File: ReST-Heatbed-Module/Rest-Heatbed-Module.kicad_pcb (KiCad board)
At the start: 2 copper layers, 25.4 x 34.2 mm, 88 parts, among them P1 02-SCREW-TERM, P2 CONN_02X03, P3 02-SCREW-TERM, P4 01X02-MALE, P5 02-SCREW-TERM, Q1 Q_BSH105, Q2 Q_AOT240L

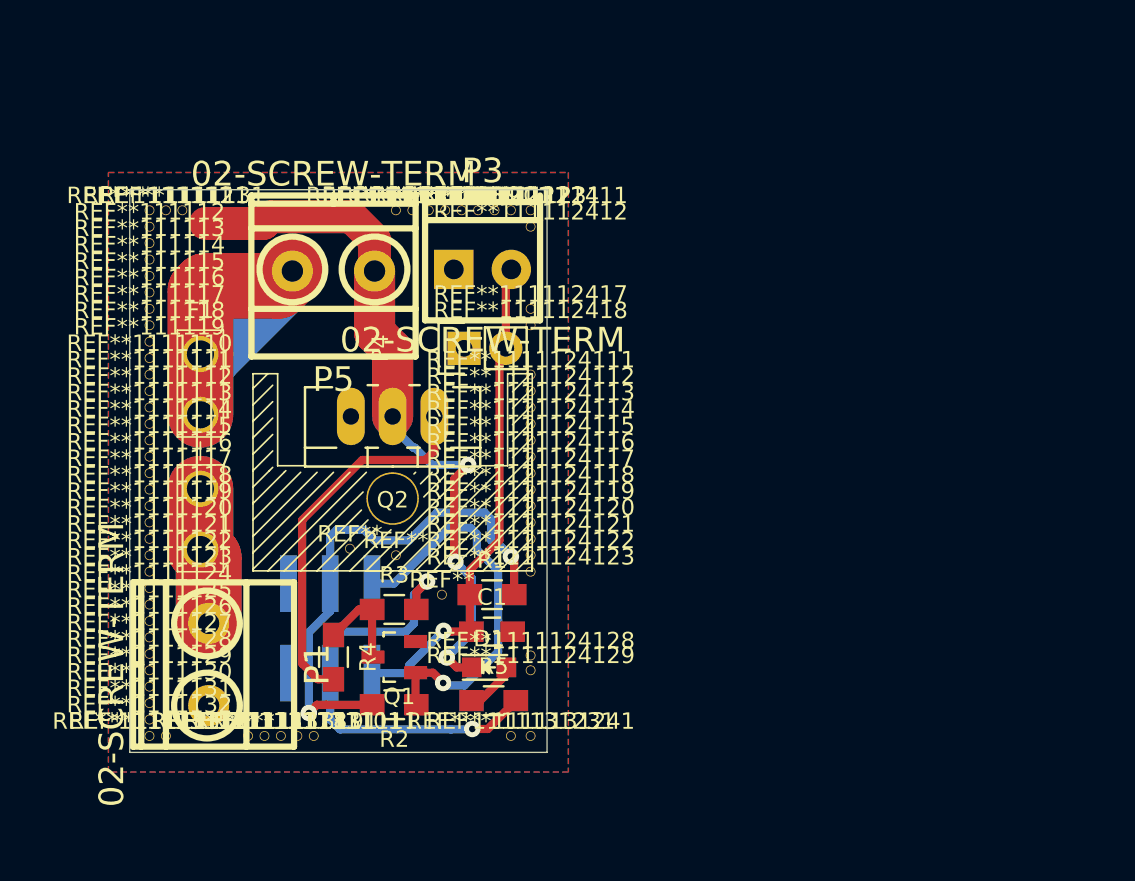
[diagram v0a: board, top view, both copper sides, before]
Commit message: Mainboard structure made and most modules finished
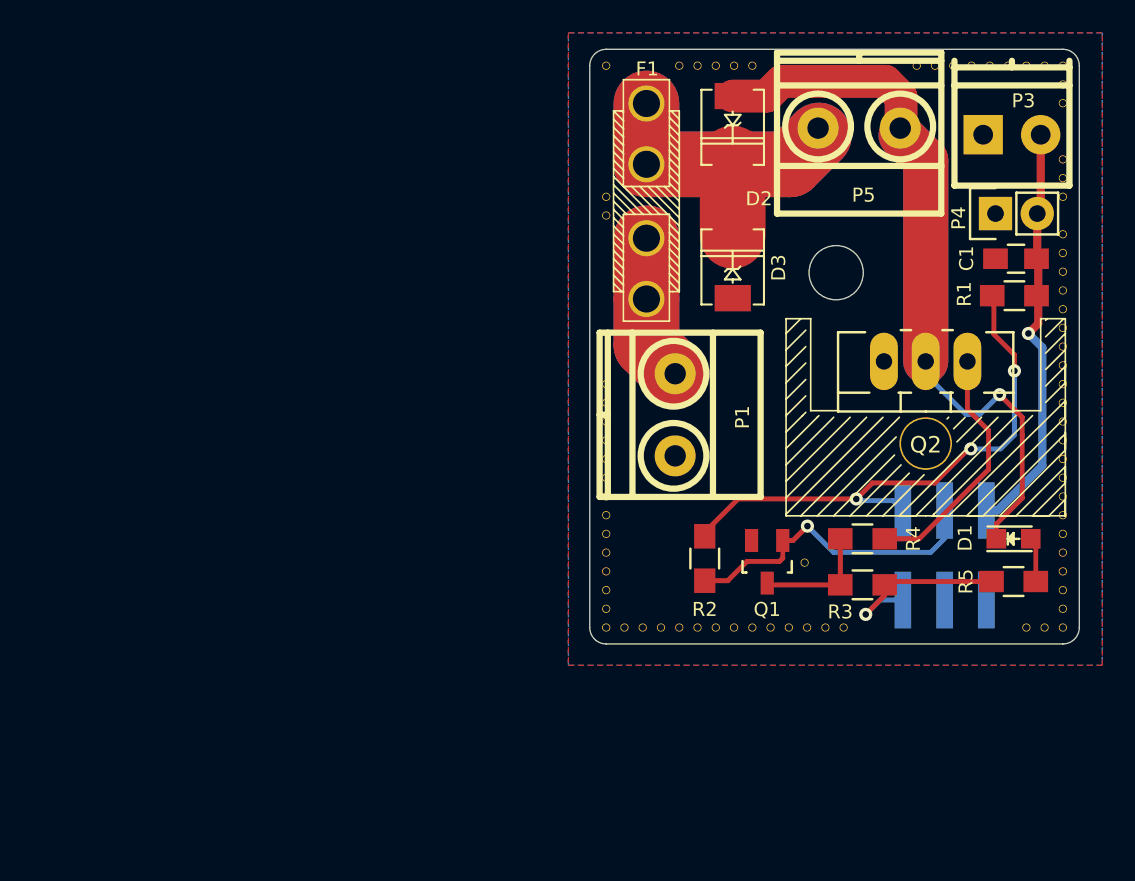
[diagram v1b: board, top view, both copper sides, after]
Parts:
- removed REF** (x3), REF**1111110, REF**1111111 (x2), REF**1111112, REF**1111113, REF**1111114, REF**1111115, REF**1111116, REF**1111117, REF**11111171 (x2), REF**1111118, REF**11111181, REF**1111119, REF**11111191, REF**111112, REF**1111120, REF**11111201, REF**1111121 (x2), REF**11111211, REF**1111122, REF**11111221, REF**1111123, REF**11111231, REF**1111124, REF**111112411, REF**1111124111, REF**1111124112, REF**1111124113, REF**1111124114, REF**1111124115, REF**1111124116, REF**1111124117, REF**1111124118, REF**1111124119, REF**111112412, REF**1111124120, REF**1111124121, REF**1111124122, REF**1111124123, REF**1111124128, REF**1111124129, REF**111112417, REF**111112418, REF**1111125, REF**1111126, REF**1111127, REF**1111128, REF**1111129, REF**111113, REF**1111130, REF**1111131 (x2), REF**1111131101, REF**111113111, REF**1111131111, REF**111113121, REF**1111131231, REF**1111131241, REF**111113171, REF**111113181, REF**111113191, REF**1111132, REF**111114, REF**111115, REF**111116, REF**111117, REF**111118, REF**111119: 1pin, ReST-Library:1pin
- added ?: , ReST-Library:1pin, F.Cu at (180.7, 88.8)
- added ?: , ReST-Library:1pin, F.Cu at (177.5, 92.8)
- added ?: , ReST-Library:1pin, F.Cu at (176.4, 92.8)
- added ?: , ReST-Library:1pin, F.Cu at (175.3, 92.8)
- added ?: , ReST-Library:1pin, F.Cu at (174.2, 92.8)
- added ?: , ReST-Library:1pin, F.Cu at (173.0, 92.8)
- added ?: , ReST-Library:1pin, F.Cu at (171.9, 92.8)
- added ?: , ReST-Library:1pin, F.Cu at (170.8, 92.8)
- added ?: , ReST-Library:1pin, F.Cu at (169.7, 92.8)
- added ?: , ReST-Library:1pin, F.Cu at (196.4, 91.7)
- added ?: , ReST-Library:1pin, F.Cu at (196.4, 90.5)
- added ?: , ReST-Library:1pin, F.Cu at (196.4, 92.8)
- added ?: , ReST-Library:1pin, F.Cu at (196.4, 89.4)
- added ?: , ReST-Library:1pin, F.Cu at (196.4, 88.2)
- added ?: , ReST-Library:1pin, F.Cu at (196.4, 87.1)
- added ?: , ReST-Library:1pin, F.Cu at (196.4, 86.0)
- added ?: , ReST-Library:1pin, F.Cu at (196.4, 84.8)
- added ?: , ReST-Library:1pin, F.Cu at (196.4, 83.7)
- added ?: , ReST-Library:1pin, F.Cu at (196.4, 82.5)
- added ?: , ReST-Library:1pin, F.Cu at (196.4, 81.4)
- added ?: , ReST-Library:1pin, F.Cu at (196.4, 80.3)
- added ?: , ReST-Library:1pin, F.Cu at (196.4, 79.1)
- added ?: , ReST-Library:1pin, F.Cu at (195.3, 92.8)
- added ?: , ReST-Library:1pin, F.Cu at (196.4, 78.0)
- added ?: , ReST-Library:1pin, F.Cu at (196.4, 76.8)
- added ?: , ReST-Library:1pin, F.Cu at (196.4, 75.7)
- added ?: , ReST-Library:1pin, F.Cu at (196.4, 74.6)
- added ?: , ReST-Library:1pin, F.Cu at (196.4, 73.4)
- added ?: , ReST-Library:1pin, F.Cu at (196.4, 72.3)
- added ?: , ReST-Library:1pin, F.Cu at (196.4, 71.1)
- added ?: , ReST-Library:1pin, F.Cu at (196.4, 70.0)
- added ?: , ReST-Library:1pin, F.Cu at (196.4, 68.9)
- added ?: , ReST-Library:1pin, F.Cu at (196.4, 66.6)
- added ?: , ReST-Library:1pin, F.Cu at (194.2, 92.8)
- added ?: , ReST-Library:1pin, F.Cu at (196.4, 65.4)
- added ?: , ReST-Library:1pin, F.Cu at (196.4, 64.3)
- added ?: , ReST-Library:1pin, F.Cu at (196.4, 60.9)
- added ?: , ReST-Library:1pin, F.Cu at (196.4, 59.7)
- added ?: , ReST-Library:1pin, F.Cu at (168.6, 92.8)
- added ?: , ReST-Library:1pin, F.Cu at (168.6, 91.7)
- added ?: , ReST-Library:1pin, F.Cu at (168.6, 90.5)
- added ?: , ReST-Library:1pin, F.Cu at (168.6, 89.4)
- added ?: , ReST-Library:1pin, F.Cu at (168.6, 88.2)
- added ?: , ReST-Library:1pin, F.Cu at (168.6, 87.1)
- added ?: , ReST-Library:1pin, F.Cu at (183.1, 92.8)
- added ?: , ReST-Library:1pin, F.Cu at (168.6, 86.0)
- added ?: , ReST-Library:1pin, F.Cu at (168.6, 84.8)
- added ?: , ReST-Library:1pin, F.Cu at (168.6, 83.7)
- added ?: , ReST-Library:1pin, F.Cu at (168.6, 82.5)
- added ?: , ReST-Library:1pin, F.Cu at (168.6, 81.4)
- added ?: , ReST-Library:1pin, F.Cu at (168.6, 80.3)
- added ?: , ReST-Library:1pin, F.Cu at (168.6, 79.1)
- added ?: , ReST-Library:1pin, F.Cu at (168.6, 78.0)
- added ?: , ReST-Library:1pin, F.Cu at (168.6, 67.7)
- added ?: , ReST-Library:1pin, F.Cu at (168.6, 66.6)
- added ?: , ReST-Library:1pin, F.Cu at (181.9, 92.8)
- added ?: , ReST-Library:1pin, F.Cu at (196.4, 58.6)
- added ?: , ReST-Library:1pin, F.Cu at (195.3, 58.6)
- added ?: , ReST-Library:1pin, F.Cu at (194.2, 58.6)
- added ?: , ReST-Library:1pin, F.Cu at (193.1, 58.6)
- added ?: , ReST-Library:1pin, F.Cu at (192.0, 58.6)
- added ?: , ReST-Library:1pin, F.Cu at (190.8, 58.6)
- added ?: , ReST-Library:1pin, F.Cu at (189.7, 58.6)
- added ?: , ReST-Library:1pin, F.Cu at (188.6, 58.6)
- added ?: , ReST-Library:1pin, F.Cu at (187.5, 58.6)
- added ?: , ReST-Library:1pin, F.Cu at (177.5, 58.6)
- added ?: , ReST-Library:1pin, F.Cu at (180.8, 92.8)
- added ?: , ReST-Library:1pin, F.Cu at (176.4, 58.6)
- added ?: , ReST-Library:1pin, F.Cu at (175.3, 58.6)
- added ?: , ReST-Library:1pin, F.Cu at (174.2, 58.6)
- added ?: , ReST-Library:1pin, F.Cu at (173.0, 58.6)
- added ?: 1pin, ReST-Library:1pin, F.Cu at (182.6, 71.2)
- added ?: , ReST-Library:1pin, F.Cu at (168.6, 58.6)
- added ?: , ReST-Library:1pin, F.Cu at (179.7, 92.8)
- added ?: , ReST-Library:1pin, F.Cu at (178.6, 92.8)
- added D2: , ReST-Library:DO-214AC.SMA, F.Cu at (176.3, 62.4)
- added D3: , ReST-Library:DO-214AC.SMA, F.Cu at (176.3, 70.8)
- C1: value 10uF -> (none)
- D1: value LED -> (none)
- P1, P3, P5: value 02-SCREW-TERM -> (none)
- P2: value CONN_02X03 -> (none)
- P4: value 01X02-MALE -> (none)
- Q1: value Q_BSH105 -> (none)
- Q2: value Q_AOT240L -> (none)
- R1: value 4.7K -> (none)
- R2, R3: value 100K -> (none)
- R4: value 22R -> (none)
- R5: value 150R -> (none)
- moved C1 39.2 mm to (193.6, 70.3), turned to 180 degrees
- moved P2 37.7 mm to (189.2, 88.4)
- moved R1 36.6 mm to (193.4, 72.6), turned to 180 degrees
- moved P4 33.4 mm to (192.3, 67.6)
- moved P3 33.3 mm to (193.3, 62.1)
- moved P5 33.2 mm to (184.0, 62.4)
- moved R4 33.0 mm to (184.2, 87.4), turned to 0 degrees
- moved D1 32.9 mm to (193.4, 87.4)
- moved Q2 32.6 mm to (188.1, 76.6)
- moved R5 32.5 mm to (193.4, 90.0), turned to 180 degrees
- moved P1 32.2 mm to (172.8, 79.8)
- moved F1 31.1 mm to (171.1, 66.8)
- moved R3 28.5 mm to (184.2, 90.2)
- moved Q1 23.4 mm to (178.4, 88.8), turned to 180 degrees
- moved R2 20.9 mm to (174.6, 88.6), turned to 90 degrees
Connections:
- P2 pad 1: /T0 -> GND
- P2 pad 2: /PWM-HEATBED -> /T0
- P2 pad 3: +5V -> GND
- P2 pad 4: +3V3 -> /PWM-HEATBED
- P2 pad 5: GND -> +5V
- P2 pad 6: GND -> +3V3
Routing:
- net Net-(D1-Pad1): track 52.7 -> 87.6 mm, vias 3 -> 1
- net +5V: track 27.9 -> 11.5 mm, vias 2 -> 1
- net +12V: track 25.0 -> 34.5 mm
- net Net-(Q2-Pad1): track 22.9 -> 15.2 mm
- net /T0: track 30.6 -> 25.4 mm
- net /PWM-HEATBED: track 23.8 -> 19.3 mm
- net +3V3: track 31.8 -> 33.8 mm, vias 2 -> 3
- net Net-(Q1-Pad3): track 5.91 -> 7.29 mm
- net Net-(F1-Pad1): track 16.8 -> 17.9 mm
- net Net-(D1-Pad2): track 3.36 -> 2.72 mm
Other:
- board size 25.4 x 34.2 mm -> 29.8 x 36.2 mm
- net class Default: via_dia 1 -> 0.8
- rule via_min_size: 0.8 -> 0.6
